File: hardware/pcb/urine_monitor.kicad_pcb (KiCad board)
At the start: 2 copper layers, 64 x 100 mm, 3 parts

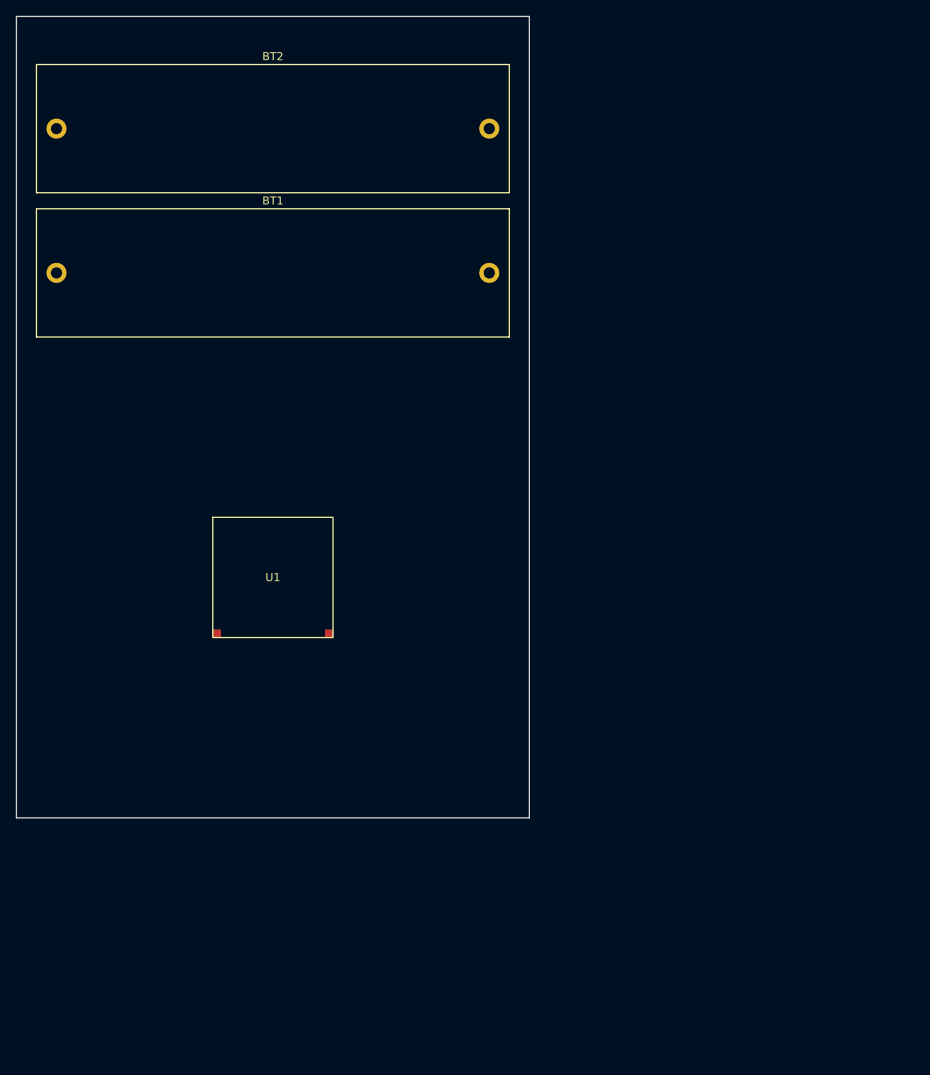
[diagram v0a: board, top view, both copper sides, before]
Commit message: init
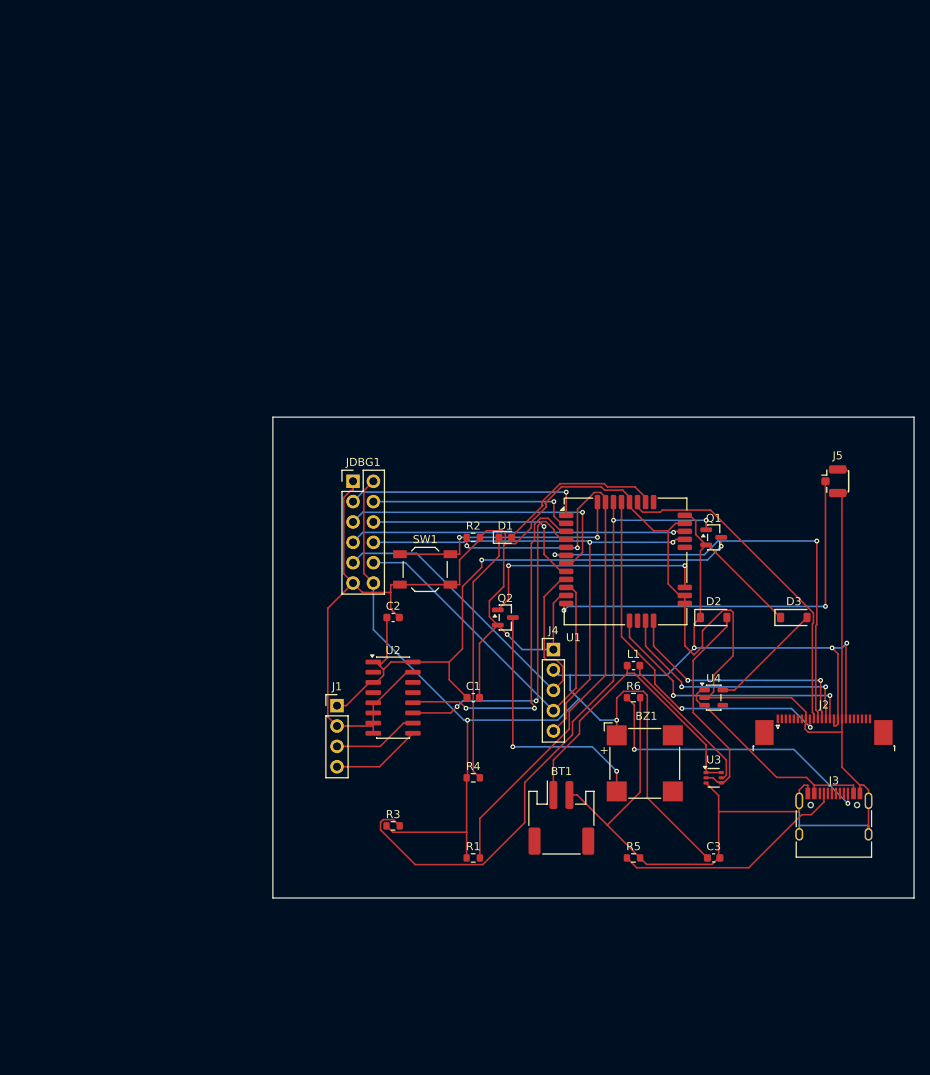
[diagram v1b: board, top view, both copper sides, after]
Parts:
- removed BT2: Keystone_1028, Project_Lib:Keystone_1028
- added BZ1: Buzzer, Buzzer_Beeper:MagneticBuzzer_CUI_CMT-8504-100-SMT, F.Cu at (46.4, 43.2)
- added C1: 10uF, Capacitor_SMD:C_0603_1608Metric, F.Cu at (25.0, 35.0)
- added C2: 0.1uF, Capacitor_SMD:C_0603_1608Metric, F.Cu at (15.0, 25.0)
- added C3: 10uF, Capacitor_SMD:C_0603_1608Metric, F.Cu at (55.0, 55.0)
- added D1: RED, LED_SMD:LED_0603_1608Metric, F.Cu at (29.0, 15.0)
- added D2: SS14, Diode_SMD:D_SOD-123, F.Cu at (55.0, 25.0)
- added D3: SS14, Diode_SMD:D_SOD-123, F.Cu at (65.0, 25.0)
- added J1: LoadCell, Connector_PinHeader_2.54mm:PinHeader_1x04_P2.54mm_Vertical, F.Cu at (8.00, 36.0)
- added J2: EInk_FPC, Connector_FFC-FPC:TE_2-1734839-4_1x24-1MP_P0.5mm_Horizontal, F.Cu at (68.8, 39.0)
- added J3: USB-C_Power, Connector_USB:USB_C_Receptacle_HRO_TYPE-C-31-M-12, F.Cu at (70.0, 51.0)
- added J4: I2C+BOOT0+PWR, Connector_PinHeader_2.54mm:PinHeader_1x05_P2.54mm_Vertical, F.Cu at (35.0, 29.0)
- added J5: Antenna_UFL, Connector_Coaxial:U.FL_Hirose_U.FL-R-SMT-1_Vertical, F.Cu at (70.0, 8.00)
- added JDBG1: DBG/SWD/I2C/UART, Connector_PinHeader_2.54mm:PinHeader_2x06_P2.54mm_Vertical, F.Cu at (10.0, 8.00)
- added L1: 4.7uH, Inductor_SMD:L_0603_1608Metric, F.Cu at (45.0, 31.0)
- added Q1: SI2301, Package_TO_SOT_SMD:SOT-23, F.Cu at (55.0, 15.0)
- added Q2: 2N7002, Package_TO_SOT_SMD:SOT-23, F.Cu at (29.0, 25.0)
- added R1: 1M, Resistor_SMD:R_0603_1608Metric, F.Cu at (25.0, 55.0)
- added R2: 1M, Resistor_SMD:R_0603_1608Metric, F.Cu at (25.0, 15.0)
- added R3: 100k, Resistor_SMD:R_0603_1608Metric, F.Cu at (15.0, 51.0)
- added R4: 1k, Resistor_SMD:R_0603_1608Metric, F.Cu at (25.0, 45.0)
- added R5: 5k1, Resistor_SMD:R_0603_1608Metric, F.Cu at (45.0, 55.0)
- added R6: 5k1, Resistor_SMD:R_0603_1608Metric, F.Cu at (45.0, 35.0)
- added SW1: USER_BTN, Button_Switch_SMD:SW_SPST_TL3342, F.Cu at (19.0, 19.0)
- added U2: HX711, Package_SO:SOIC-16_3.9x9.9mm_P1.27mm, F.Cu at (15.0, 35.0)
- added U3: TPS61220, Package_TO_SOT_SMD:SOT-363_SC-70-6, F.Cu at (55.0, 45.0)
- added U4: MIC5504-3.3, Package_TO_SOT_SMD:SOT-23-5, F.Cu at (55.0, 35.0)
- BT1: value Keystone_1028 -> BAT_JST; footprint Project_Lib:Keystone_1028 -> Connector_JST:JST_PH_S2B-PH-SM4-TB_1x02-1MP_P2.00mm_Horizontal
- U1: value (none) -> RAK3172; footprint RAK3172_Placeholder -> RF_Module:RAK3172
- moved BT1 76.9 mm to (36.0, 50.0)
- moved U1 44.0 mm to (44.0, 18.0)
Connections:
- BT1 pad 1: VCC -> BAT
- BT1 pad 2: /LINK -> GND
- U1 pad 1: GND -> UART2_RX
- U1 pad 32: VCC -> BTN_USER
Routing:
- net GND: track 0.00 -> 333.7 mm, vias 0 -> 1
- net VCC: track 0.00 -> 211.1 mm, vias 0 -> 5
- net HX_GATE: track 0.00 -> 83.1 mm, vias 0 -> 2
- net HX_VCC: track 0.00 -> 76.2 mm, vias 0 -> 2
- net BAT_SENSE: track 0.00 -> 75.9 mm, vias 0 -> 2
- net BOOT0: track 0.00 -> 64.6 mm, vias 0 -> 2
- net EINK_DC: track 0.00 -> 57.2 mm, vias 0 -> 2
- net I2C_SCL: track 0.00 -> 50.1 mm
- net RF: track 0.00 -> 49.4 mm, vias 0 -> 2
- net I2C_SDA: track 0.00 -> 47.5 mm
- net EINK_BUSY: track 0.00 -> 47.1 mm, vias 0 -> 2
- net HX711_DT: track 0.00 -> 43.8 mm, vias 0 -> 2
- net HX711_SCK: track 0.00 -> 42.8 mm, vias 0 -> 2
- net NRST: track 0.00 -> 42.0 mm, vias 0 -> 1
- net EINK_RST: track 0.00 -> 41.6 mm
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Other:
- board size 64 x 100 mm -> 80 x 60 mm

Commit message: init
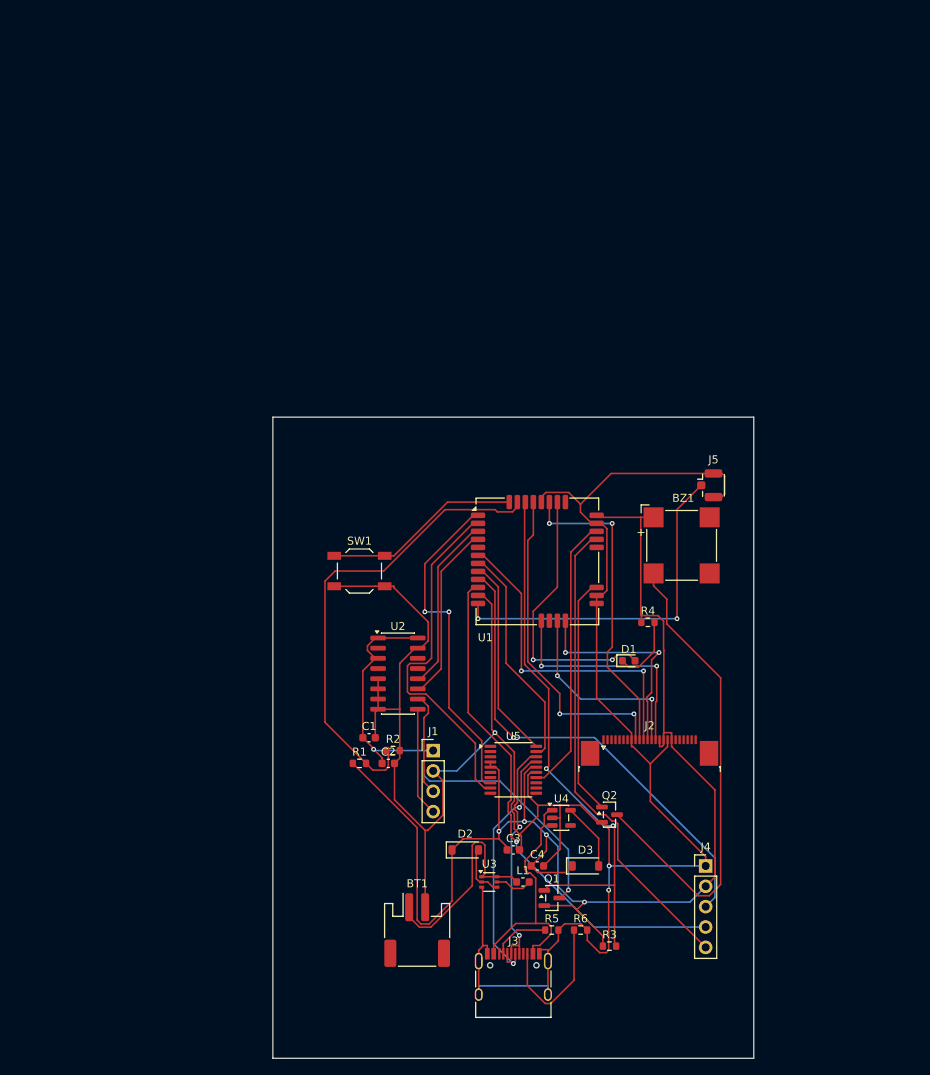
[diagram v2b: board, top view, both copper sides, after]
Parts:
- removed JDBG1: DBG/SWD/I2C/UART, Connector_PinHeader_2.54mm:PinHeader_2x06_P2.54mm_Vertical
- added C4: 0.1uF, Capacitor_SMD:C_0603_1608Metric, F.Cu at (33.0, 56.0)
- added U5: STM32F042F6P6 (USB CDC + CMSIS-DAP), Package_SO:TSSOP-20_4.4x6.5mm_P0.65mm, F.Cu at (30.0, 44.0)
- J3: value USB-C_Power -> USB-C_Dev
- moved Q1 49.3 mm to (34.8, 60.0)
- moved J3 44.7 mm to (30.0, 71.0)
- moved D2 42.4 mm to (24.0, 54.0)
- moved D3 40.5 mm to (39.0, 56.0)
- moved J4 33.0 mm to (54.0, 56.0)
- moved R3 30.9 mm to (42.0, 66.0)
- moved U3 30.9 mm to (27.0, 58.0)
- moved L1 30.3 mm to (31.2, 58.0)
- moved R6 29.7 mm to (38.4, 64.0)
- moved R4 29.2 mm to (46.8, 25.6)
- moved R2 28.4 mm to (15.0, 41.6)
- moved Q2 27.8 mm to (42.0, 49.6)
- moved BZ1 27.6 mm to (51.0, 16.0)
- moved C3 25.0 mm to (30.0, 54.0)
- moved U4 24.2 mm to (36.0, 50.0)
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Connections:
- J3 pad A6: (no net) -> USB_DP
- J3 pad A7: (no net) -> USB_DM
- J3 pad B6: (no net) -> USB_DP
- J3 pad B7: (no net) -> USB_DM
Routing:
- net USB_DM: track 0.00 -> 32.4 mm, vias 0 -> 2
- net VCC: track 211.1 -> 180.8 mm, vias 5 -> 4
- net USB_DP: track 0.00 -> 29.3 mm, vias 0 -> 2
- net GND: track 333.7 -> 306.4 mm, vias 1 -> 3
- net BUZZ_SINK: track 32.9 -> 60.0 mm, vias 2 -> 0
- net LED_NET: track 31.7 -> 8.76 mm
- net CC1: track 29.6 -> 7.19 mm
- net HX711_DT: track 43.8 -> 22.1 mm, vias 2 -> 0
- net HX711_SCK: track 42.8 -> 22.4 mm, vias 2 -> 0
- net U3_OUT: track 27.0 -> 6.71 mm
- net CC2: track 37.5 -> 18.2 mm, vias 2 -> 0
- net UART2_TX: track 26.2 -> 44.2 mm, vias 1 -> 0
- net BAT_SENSE: track 75.9 -> 59.0 mm, vias 2 -> 0
- net I2C_SDA: track 47.5 -> 64.0 mm, vias 0 -> 1
- net EINK_DC: track 57.2 -> 40.9 mm
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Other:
- board size 80 x 60 mm -> 60 x 80 mm
